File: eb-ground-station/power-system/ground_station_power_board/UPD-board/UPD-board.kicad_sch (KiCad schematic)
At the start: 100 parts, among them J1 Conn_01x04, J10 PI 1827486, J11 PC 1720806, J12 Conn_02x02_Odd_Even, J13 Conn_01x05, J14 Conn_01x04, J2 Conn_01x03, J3 Conn_01x03, J4 Conn_01x03, J5 Conn_01x03, J6 Conn_01x03, J7 PI 1924143, J8 PI 1827923, J9 PI 1827486, Q21 SUD50P08-25L-E3, Q22 SUD50P08-25L-E3, U1 MAX7310, U2 MAX7310, U3 MAX7310, U4 ADT7410TRZ, U5 ADS1115IDGS, U6 UA78M33, U7 U_RasPi_40pin

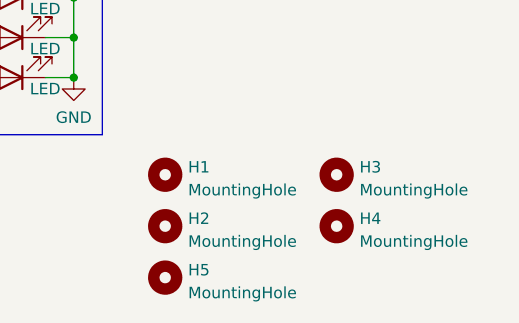
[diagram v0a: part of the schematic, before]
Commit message: UPD board is ready for production I think
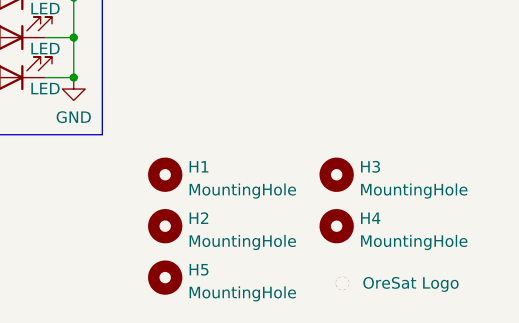
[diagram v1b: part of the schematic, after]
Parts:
- added LOGO1: OreSat Logo, oresat-footprints:logo-small, symbol graphics:dot_small
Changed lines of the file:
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@@
     (pin "2")
   )
-  (symbol (lib_id "graphics:dot_small") (at 186.69 195.58 0) (unit 1)
+  (symbol (lib_name "dot_small_8") (lib_id "graphics:dot_small") (at 186.69 195.58 0) (unit 1)
     (in_bom no) (on_board no) (fields_autoplaced)
     (property "Reference" "#SIM6" (id 0) (at 186.69 195.58 0)
@@
     (pin "1")
   )
-  (symbol (lib_id "graphics:dot_small") (at 152.4 148.59 0) (unit 1)
+  (symbol (lib_name "dot_small_4") (lib_id "graphics:dot_small") (at 152.4 148.59 0) (unit 1)
     (in_bom no) (on_board no) (fields_autoplaced)
     (property "Reference" "#SIM4" (id 0) (at 152.4 148.59 0)
@@
     (pin "8")
   )
-  (symbol (lib_id "graphics:dot_small") (at 152.4 107.95 0) (unit 1)
+  (symbol (lib_name "dot_small_3") (lib_id "graphics:dot_small") (at 152.4 107.95 0) (unit 1)
     (in_bom no) (on_board no) (fields_autoplaced)
     (property "Reference" "#SIM3" (id 0) (at 152.4 107.95 0)
@@
     (pin "2")
   )
-  (symbol (lib_id "graphics:dot_small") (at 190.5 191.77 0) (unit 1)
+  (symbol (lib_name "dot_small_6") (lib_id "graphics:dot_small") (at 190.5 191.77 0) (unit 1)
     (in_bom no) (on_board no) (fields_autoplaced)
     (property "Reference" "#SIM7" (id 0) (at 190.5 191.77 0)
@@
     (pin "1")
   )
-  (symbol (lib_id "graphics:dot_small") (at 223.52 195.58 0) (unit 1)
+  (symbol (lib_name "dot_small_9") (lib_id "graphics:dot_small") (at 223.52 195.58 0) (unit 1)
     (in_bom no) (on_board no) (fields_autoplaced)
     (property "Reference" "#SIM8" (id 0) (at 223.52 195.58 0)
@@
     (pin "1")
   )
-  (symbol (lib_id "graphics:dot_small") (at 152.4 199.39 0) (unit 1)
+  (symbol (lib_name "dot_small_2") (lib_id "graphics:dot_small") (at 152.4 199.39 0) (unit 1)
     (in_bom no) (on_board no) (fields_autoplaced)
     (property "Reference" "#SIM1" (id 0) (at 152.4 199.39 0)
@@
   (symbol (lib_id "power:GND") (at 177.8 35.56 0) (unit 1)
     (in_bom yes) (on_board yes)
-    (property "Reference" "#PWR?" (id 0) (at 177.8 41.91 0)
+    (property "Reference" "#PWR0109" (id 0) (at 177.8 41.91 0)
       (effects (font (size 1.27 1.27)) hide)
     )
@@
     (pin "3")
   )
-  (symbol (lib_id "graphics:dot_small") (at 182.88 199.39 0) (unit 1)
+  (symbol (lib_name "dot_small_7") (lib_id "graphics:dot_small") (at 182.88 199.39 0) (unit 1)
     (in_bom no) (on_board no) (fields_autoplaced)
     (property "Reference" "#SIM5" (id 0) (at 182.88 199.39 0)
@@
     (pin "2")
   )
-  (symbol (lib_id "graphics:dot_small") (at 152.4 62.23 0) (unit 1)
+  (symbol (lib_name "dot_small_5") (lib_id "graphics:dot_small") (at 152.4 62.23 0) (unit 1)
     (in_bom no) (on_board no) (fields_autoplaced)
     (property "Reference" "#SIM2" (id 0) (at 152.4 62.23 0)
@@
     (pin "2")
   )
+  (symbol (lib_name "dot_small_1") (lib_id "graphics:dot_small") (at 402.59 259.08 0) (unit 1)
+    (in_bom no) (on_board yes)
+    (property "Reference" "LOGO1" (id 0) (at 402.59 259.08 0)
+      (effects (font (size 1.27 1.27)) hide)
+    )
+    (property "Value" "OreSat Logo" (id 1) (at 410.21 259.08 0))
+    (property "Footprint" "oresat-footprints:logo-small" (id 2) (at 402.59 259.08 0)
+      (effects (font (size 1.27 1.27)) hide)
+    )
+    (property "Datasheet" "" (id 3) (at 402.59 259.08 0)
+      (effects (font (size 1.27 1.27)) hide)
+    )
+  )
   (symbol (lib_id "Graphic:SYM_Arrow_Normal") (at 90.17 109.22 90) (unit 1)
     (in_bom yes) (on_board no) (fields_autoplaced)
@@
       (reference "#PWR0108") (unit 1) (value "+5V") (footprint "")
     )
+    (path "/d5a3a6f9-2ee9-4bcb-b545-e0c83ae3c111"
+      (reference "#PWR0109") (unit 1) (value "GND") (footprint "")
+    )
     (path "/3a1c5476-bb6a-4918-80d3-82e1846e9dbb/84c28457-6e31-4c65-8539-377808b3bd60"
       (reference "#PWR0111") (unit 1) (value "GND") (footprint "")
@@
       (reference "#PWR0137") (unit 1) (value "+12V") (footprint "")
     )
-    (path "/d5a3a6f9-2ee9-4bcb-b545-e0c83ae3c111"
-      (reference "#PWR?") (unit 1) (value "GND") (footprint "")
-    )
     (path "/ad5194cd-faa1-48ea-8b7b-4ebe86ba3152"
       (reference "#SIM1") (unit 1) (value "dot_small") (footprint "")
@@
       (reference "JP29") (unit 1) (value "SolderJumper-HP") (footprint "oresat-footprints:JP-SOLDER-2way-HP")
     )
+    (path "/fd8cf496-8078-42c7-846c-0a70693744f4"
+      (reference "LOGO1") (unit 1) (value "OreSat Logo") (footprint "oresat-footprints:logo-small")
+    )
     (path "/3a1c5476-bb6a-4918-80d3-82e1846e9dbb/6f338c88-571d-40d4-a656-bab0f745db42"
